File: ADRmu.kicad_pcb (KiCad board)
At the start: 4 copper layers, 160 x 100 mm, 41 parts, among them J1 DIN41612_02x16_AC_EvenPins, J10 Conn_01x01, J11 Conn_01x01, J12 Conn_01x01, J2 Conn_01x01, J3 Conn_01x01, J4 Conn_01x01, J5 Conn_01x01, J6 Conn_01x01, J7 Conn_01x01, J8 Conn_01x01, J9 Conn_01x01, Q1 Q_NPN_BCE, U1 L78L33_SOT89, U2 TMP117, U3 LT3439, U4 ADR1000, U5 Opamp_Dual

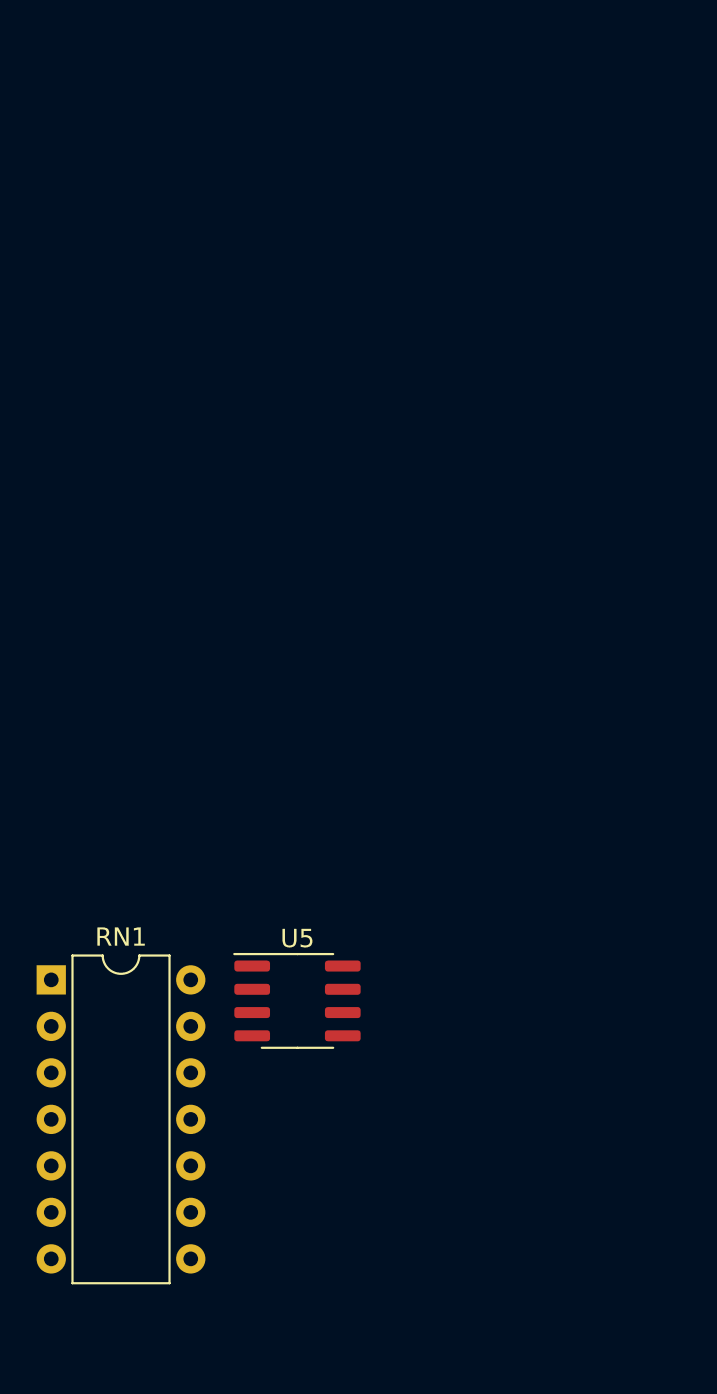
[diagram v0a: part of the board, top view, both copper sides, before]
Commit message: asdf
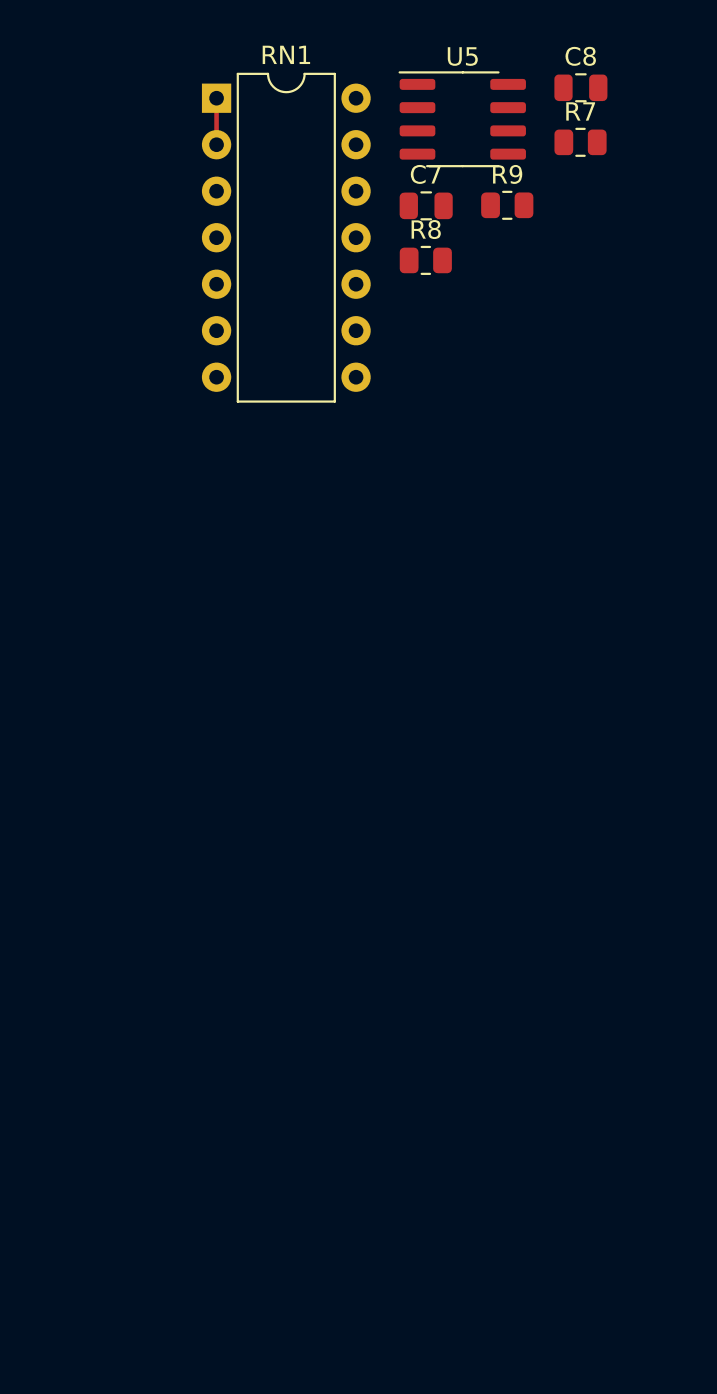
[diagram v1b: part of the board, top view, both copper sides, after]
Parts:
- added C7: 100n, Capacitor_SMD:C_0805_2012Metric, F.Cu at (45.7, 55.9)
- added C8: 100n, Capacitor_SMD:C_0805_2012Metric, F.Cu at (54.2, 49.4)
- added R7: 1k, Resistor_SMD:R_0805_2012Metric, F.Cu at (54.1, 52.4)
- added R8: 1M, Resistor_SMD:R_0805_2012Metric, F.Cu at (45.7, 58.9)
- added R9: 10k, Resistor_SMD:R_0805_2012Metric, F.Cu at (50.1, 55.9)
- moved U5 49.0 mm to (47.7, 51.1)
- moved RN1 49.0 mm to (34.3, 50.0)
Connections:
- D3 pad 1: unconnected-(D3-Pad1) -> /ref/GNDf
- Q1 pad 1: unconnected-(Q1-Pad1) -> Net-(Q1-Pad1)
- Q1 pad 2: unconnected-(Q1-Pad2) -> /ref/12Vf
- RN1 pad 11: Net-(U4-Pad6) -> /ref/ADR_Pin6
- RN1 pad 12: Net-(U4-Pad7) -> Net-(C8-Pad1)
- RN1 pad 13: Net-(U4-Pad5) -> /ref/ADR_Pin8
- RN1 pad 14: Net-(U4-Pad8) -> Net-(RN1-Pad14)
- RN1 pad 4: Net-(U4-Pad7) -> /ref/ADR_Pin6
- RN1 pad 7: unconnected-(RN1-Pad7) -> Net-(RN1-Pad7)
- RN1 pad 9: unconnected-(RN1-Pad9) -> Net-(RN1-Pad7)
- U4 pad 5: Net-(U4-Pad5) -> Net-(RN1-Pad14)
- U4 pad 6: Net-(U4-Pad6) -> /ref/ADR_Pin6
- U4 pad 7: Net-(U4-Pad7) -> Net-(C8-Pad1)
- U4 pad 8: Net-(U4-Pad8) -> /ref/ADR_Pin8
- U5 pad 5: unconnected-(U5-Pad5) -> /ref/ADR_Pin8
- U5 pad 6: unconnected-(U5-Pad6) -> Net-(R8-Pad2)
- U5 pad 7: unconnected-(U5-Pad7) -> Net-(R7-Pad2)
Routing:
- net Net-(D4-Pad1): track 0.00 -> 2.54 mm
